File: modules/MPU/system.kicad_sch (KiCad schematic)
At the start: 2 parts, among them J1 CardConnector

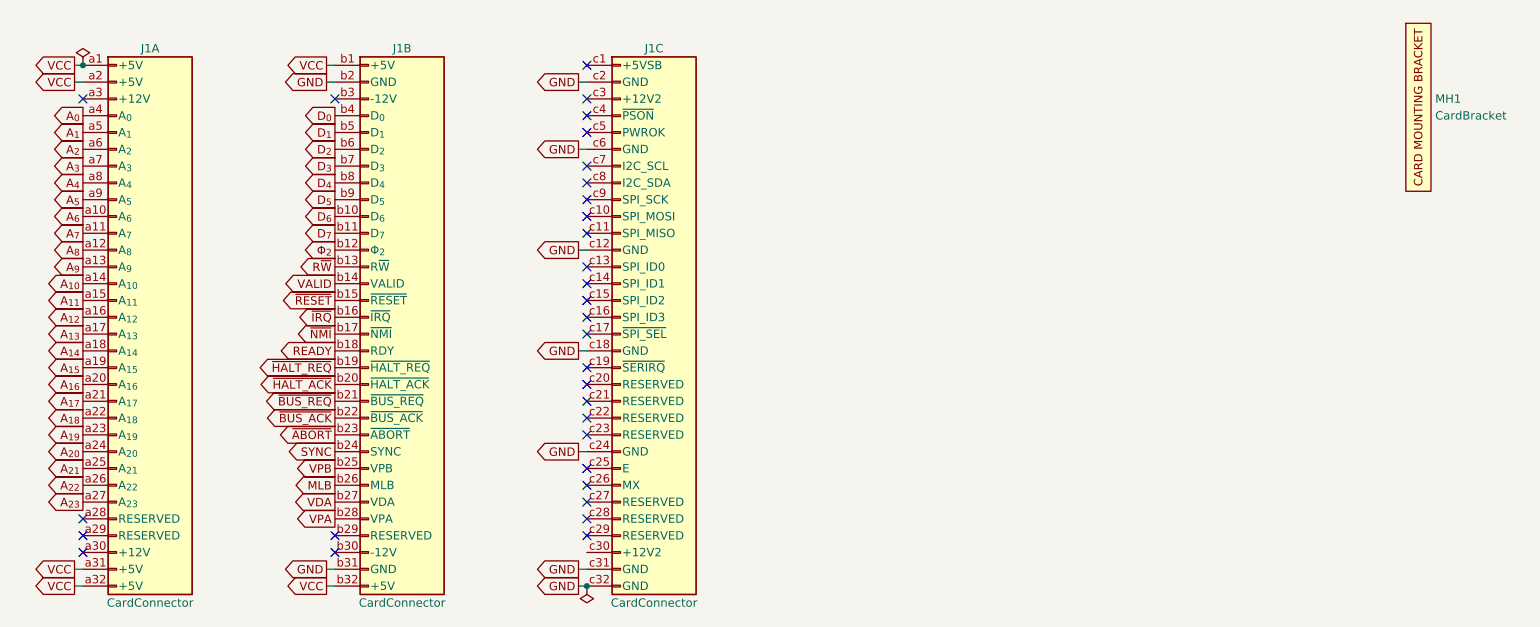
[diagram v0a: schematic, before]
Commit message: minor PW PCB tweaks
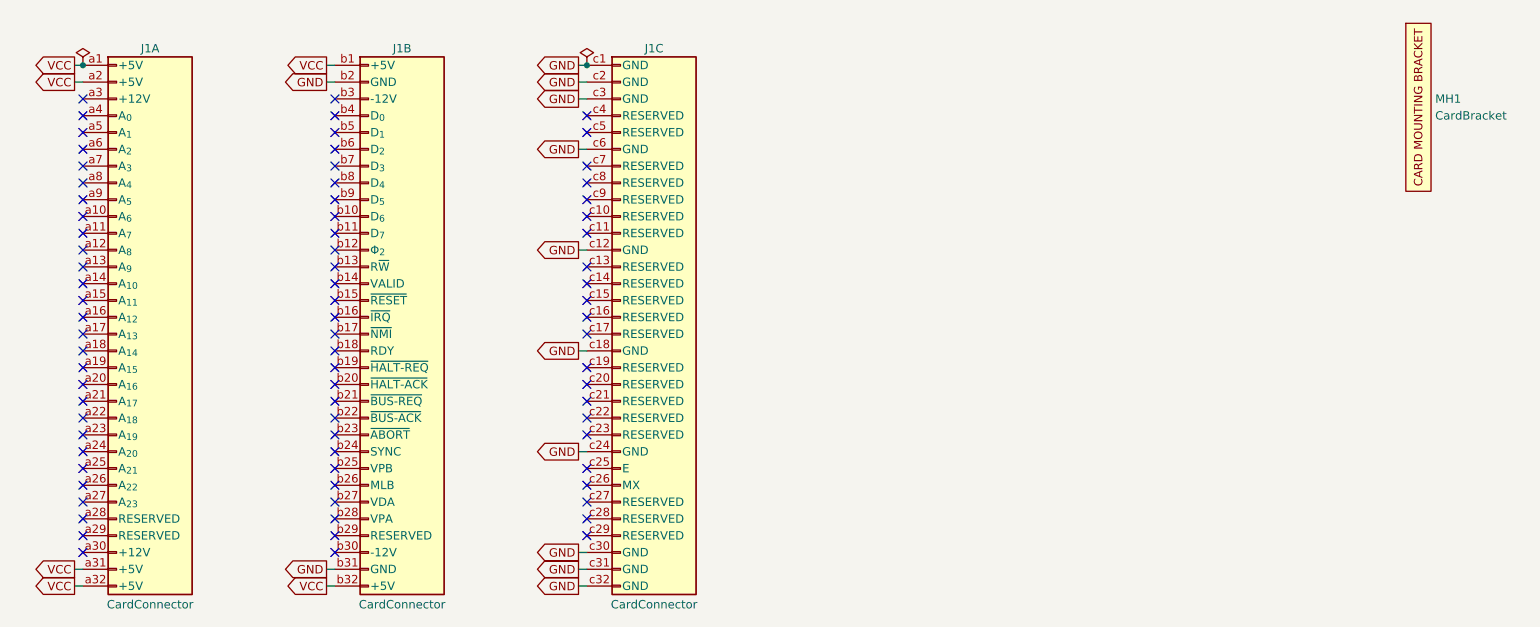
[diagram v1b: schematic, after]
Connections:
- net GND: now also J1.c1 (GND), J1.c3 (GND), J1.c30 (GND)
- net A_{0}: no longer names the net of J1.a4 (A_{0})
- net A_{10}: no longer names the net of J1.a14 (A_{10})
- net A_{11}: no longer names the net of J1.a15 (A_{11})
- net A_{12}: no longer names the net of J1.a16 (A_{12})
- net A_{13}: no longer names the net of J1.a17 (A_{13})
- net A_{14}: no longer names the net of J1.a18 (A_{14})
- net A_{15}: no longer names the net of J1.a19 (A_{15})
- net A_{16}: no longer names the net of J1.a20 (A_{16})
- net A_{17}: no longer names the net of J1.a21 (A_{17})
- net A_{18}: no longer names the net of J1.a22 (A_{18})
- net A_{19}: no longer names the net of J1.a23 (A_{19})
- net A_{1}: no longer names the net of J1.a5 (A_{1})
- net A_{20}: no longer names the net of J1.a24 (A_{20})
- net A_{21}: no longer names the net of J1.a25 (A_{21})
- net A_{22}: no longer names the net of J1.a26 (A_{22})
- net A_{23}: no longer names the net of J1.a27 (A_{23})
- net A_{2}: no longer names the net of J1.a6 (A_{2})
- net A_{3}: no longer names the net of J1.a7 (A_{3})
- net A_{4}: no longer names the net of J1.a8 (A_{4})
- net A_{5}: no longer names the net of J1.a9 (A_{5})
- net A_{6}: no longer names the net of J1.a10 (A_{6})
- net A_{7}: no longer names the net of J1.a11 (A_{7})
- net A_{8}: no longer names the net of J1.a12 (A_{8})
- net A_{9}: no longer names the net of J1.a13 (A_{9})
- net D_{0}: no longer names the net of J1.b4 (D_{0})
- net D_{1}: no longer names the net of J1.b5 (D_{1})
- net D_{2}: no longer names the net of J1.b6 (D_{2})
- net D_{3}: no longer names the net of J1.b7 (D_{3})
- net D_{4}: no longer names the net of J1.b8 (D_{4})
- net D_{5}: no longer names the net of J1.b9 (D_{5})
- net D_{6}: no longer names the net of J1.b10 (D_{6})
- net D_{7}: no longer names the net of J1.b11 (D_{7})
- net MLB: no longer names the net of J1.b26 (MLB)
- net READY: no longer names the net of J1.b18 (RDY)
- net R~{W}: no longer names the net of J1.b13 (R~{W})
- net SYNC: no longer names the net of J1.b24 (SYNC)
- net VALID: no longer names the net of J1.b14 (VALID)
- net VDA: no longer names the net of J1.b27 (VDA)
- net VPA: no longer names the net of J1.b28 (VPA)
- net VPB: no longer names the net of J1.b25 (VPB)
- net ~{ABORT}: no longer names the net of J1.b23 (~{ABORT})
- net ~{BUS_ACK}: no longer names the net of J1.b22 (~{BUS-ACK})
- net ~{BUS_REQ}: no longer names the net of J1.b21 (~{BUS-REQ})
- net ~{HALT_ACK}: no longer names the net of J1.b20 (~{HALT-ACK})
- net ~{HALT_REQ}: no longer names the net of J1.b19 (~{HALT-REQ})
- net ~{IRQ}: no longer names the net of J1.b16 (~{IRQ})
- net ~{NMI}: no longer names the net of J1.b17 (~{NMI})
- net ~{RESET}: no longer names the net of J1.b15 (~{RESET})
- net Φ_{2}: no longer names the net of J1.b12 (Φ_{2})
- no-connect marks 31 -> 78
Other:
- title: BLA-65 -> MPU-65
- moved on the sheet: J1C
